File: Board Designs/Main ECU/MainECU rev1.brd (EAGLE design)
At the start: 120.6 x 78.9 mm, 144 parts, among them X1 CONNECTOR-37, X2 CONNECTOR-4AUTOSPORT, X3 CONNECTOR-4NANO-FIT-VERTICAL-4, X4 CONNECTOR-4NANO-FIT-VERTICAL-4

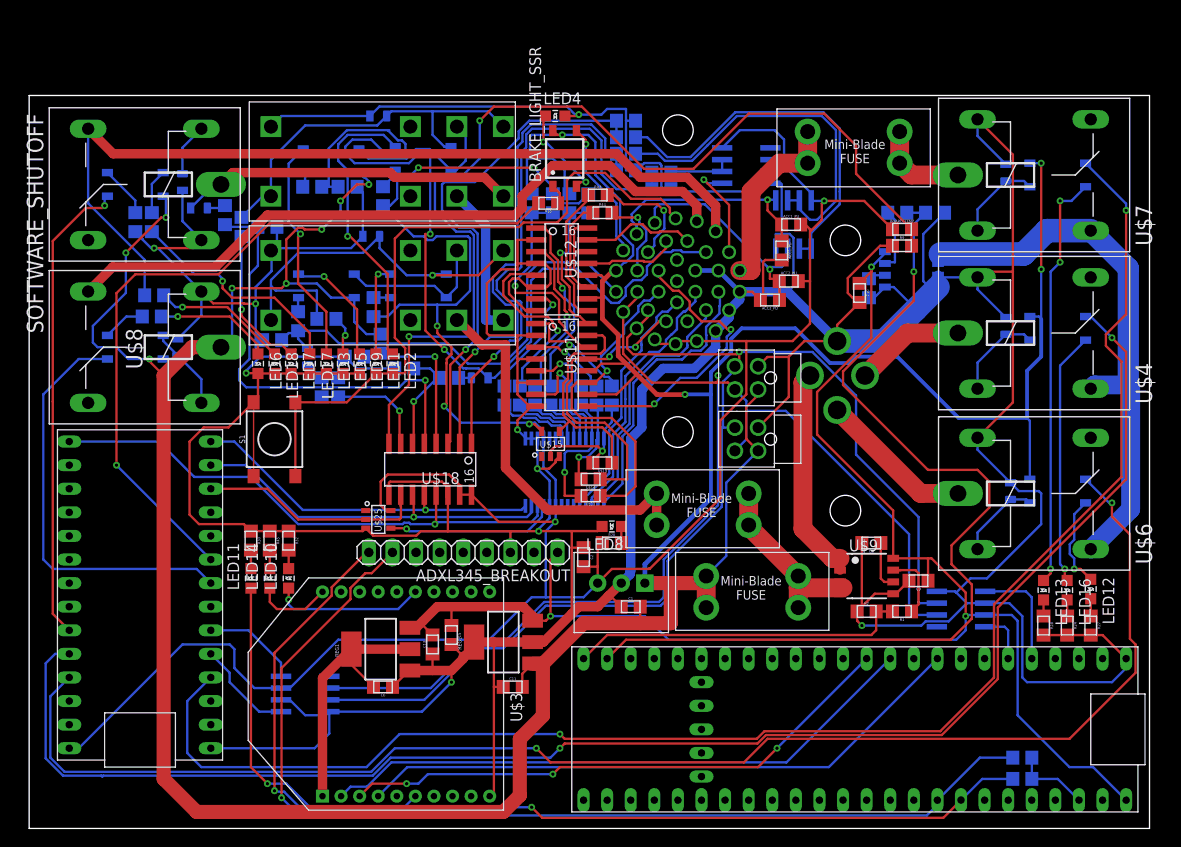
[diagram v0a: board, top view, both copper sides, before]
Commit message: Updated Rev 2 Schematic/Rev 1 Layout
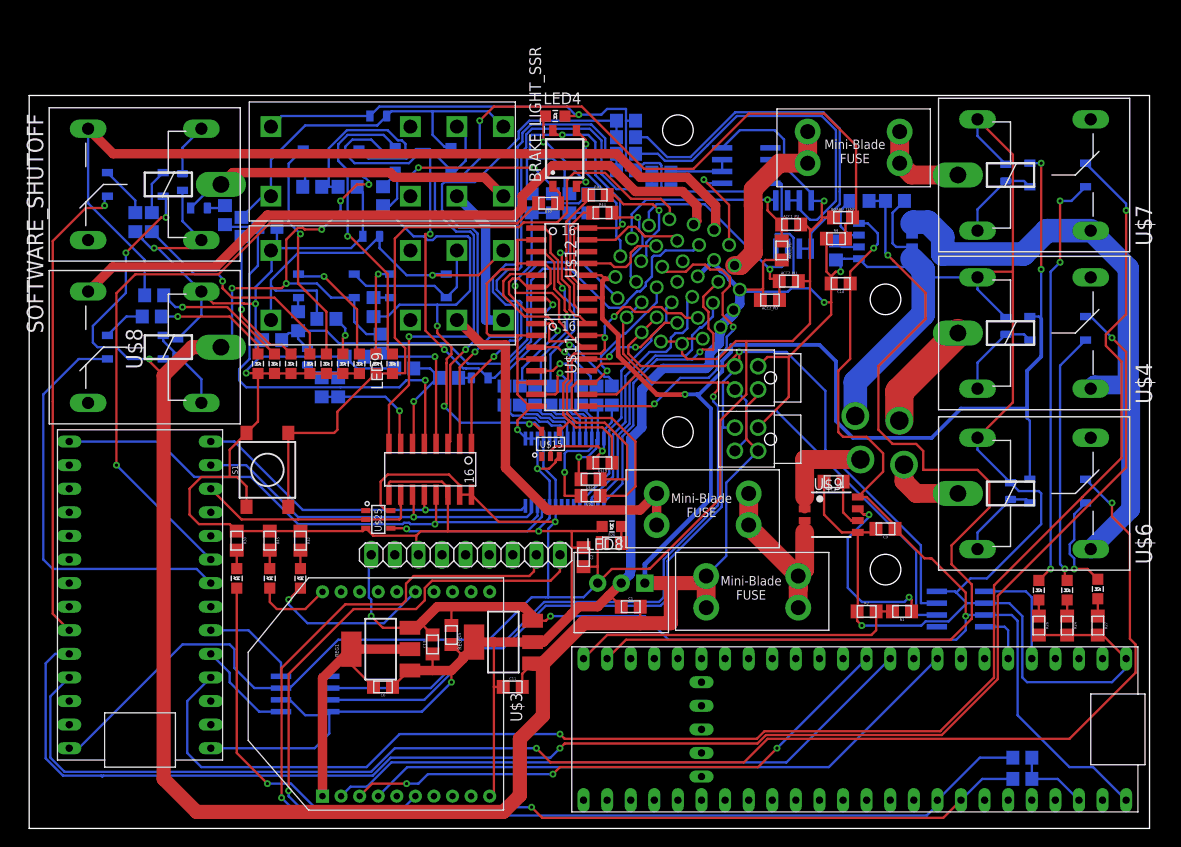
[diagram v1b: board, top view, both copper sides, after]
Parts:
- moved C8 7.75 mm to (93.0, 36.8)
- moved X2 7.68 mm to (98.6, 41.9), turned to 225 degrees
- moved U$9 7.62 mm to (92.7, 33.3)
- moved R9 7.15 mm to (93.2, 63.0)
- moved C9 6.62 mm to (98.6, 31.8)
- moved BOARD_TEMP 6.48 mm to (94.0, 65.3)
- moved C7 5.40 mm to (93.2, 61.7)
- moved R4 4.50 mm to (99.6, 67.1)
- moved R3 4.26 mm to (95.8, 67.1)
- moved U$10 4.13 mm to (98.6, 62.7)
- moved S1 3.39 mm to (32.0, 38.1)
- moved ADXL345_BREAKOUT 2.30 mm to (52.1, 29.0), turned to 0 degrees
- moved C10 2.27 mm to (93.7, 58.2), turned to 180 degrees
- moved LED11 1.52 mm to (28.7, 26.4)
- moved R30 1.52 mm to (28.7, 30.5)
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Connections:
- removed net DFASH_IO8: X1.P$28
- net +12V: now also X1.P$7; no longer X1.P$9
- net +5V: now also X1.P$11, X1.P$12; no longer X1.P$14, X1.P$15
- net BMS_OK: now also X1.P$19; no longer X1.P$20
- net BRAKE_LIGHT: now also X1.P$6; no longer X1.P$8
- net CANH: now also X1.P$10, X1.P$25; no longer X1.P$12, X1.P$26
- net CANL: now also X1.P$24, X1.P$9; no longer X1.P$11, X1.P$25
- net DASH_CTRL10: now also X1.P$28; no longer X1.P$29
- net DASH_CTRL11: now also X1.P$35; no longer X1.P$36
- net DASH_CTRL12: now also X1.P$34; no longer X1.P$35
- net DASH_CTRL9: now also X1.P$29; no longer X1.P$30
- net DASH_IO1: now also X1.P$22; no longer X1.P$23
- net DASH_IO2: now also X1.P$23; no longer X1.P$24
- net DASH_IO3: now also X1.P$21; no longer X1.P$22
- net DASH_IO4: now also X1.P$20; no longer X1.P$21
- net DASH_IO5: now also X1.P$32; no longer X1.P$33
- net DASH_IO6: now also X1.P$33; no longer X1.P$34
- net DASH_IO7: now also X1.P$26; no longer X1.P$27
- net DASH_IO8: now also X1.P$27
- net GND: now also X1.P$14, X1.P$15, X1.P$30, X1.P$36; no longer X1.P$17, X1.P$18, X1.P$19, X1.P$31
- net INVERTER_SUPPLY: now also X1.P$2; no longer X1.P$4
- net LATCH_EXT_BUTTON: now also X1.P$3; no longer X1.P$5
- net N$1: now also X1.P$17; no longer X1.P$1
- net OKHS: now also X1.P$8; no longer X1.P$10
- net SHUTDOWN_D: now also X1.P$1; no longer X1.P$3
- net SIGNAL_ACCEL1: now also X1.P$5; no longer X1.P$7
- net SIGNAL_ACCEL2: now also X1.P$4; no longer X1.P$6
- net SIGNAL_BRAKE: now also X1.P$18; no longer X1.P$2
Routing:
- net SCL: track 112.8 -> 130.5 mm
- net SDA: track 114.2 -> 130.8 mm
- net DASH_IO8: track 24.4 -> 37.5 mm, vias 0 -> 2
- net 12VIN: track 23.4 -> 11.3 mm
- net N$3: track 7.42 -> 19.4 mm, vias 0 -> 2
- net PUMP1-: track 16.7 -> 8.14 mm
- net GND: track 724.6 -> 730.3 mm, vias 9 -> 11
- net CURRENTSENSE2: track 60.9 -> 66.3 mm
- net DASH_IO5: track 31.1 -> 35.4 mm
- net TELEMETRY5V: track 163.6 -> 167.8 mm, vias 3 -> 4
- net +5V: track 296.5 -> 292.7 mm
- net LATCH_EXT_BUTTON: track 73.6 -> 76.7 mm
- net TEMPSENSE: track 109.9 -> 107.1 mm
- net CANL: track 129.9 -> 127.2 mm
- net DASH_CTRL9: track 30.5 -> 33.1 mm, vias 0 -> 1
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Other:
- board text added: "Assoc"
- board text added: "BMS OK"
- board text added: "BMSCoil"
- board text added: "Designed By Parker Jones"
- board text added: "Fan1"
- board text added: "Fan2"
- board text added: "HyTech 2019 Main ECU rev1"
- board text added: "IMD Coil"
- board text added: "IMDOK"
- board text added: "Inverter"
- board text added: "Latch Button"
- board text added: "MQTT"
- board text added: "PUMP"
- board text added: "Shutdown"
- board text added: "Software"
